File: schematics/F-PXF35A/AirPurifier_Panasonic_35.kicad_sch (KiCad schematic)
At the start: 63 parts, among them Q1 N6, Q2 N6, Q3 N6, Q4 N6, Q5 N6, Q7 N6, SW1 ON/OFF, SW2 AirVolume, SW3 Turbo, SW4 Sleep, U1 WEMOS_D1_mini, U2 PCF8575DBR, U3 PC847

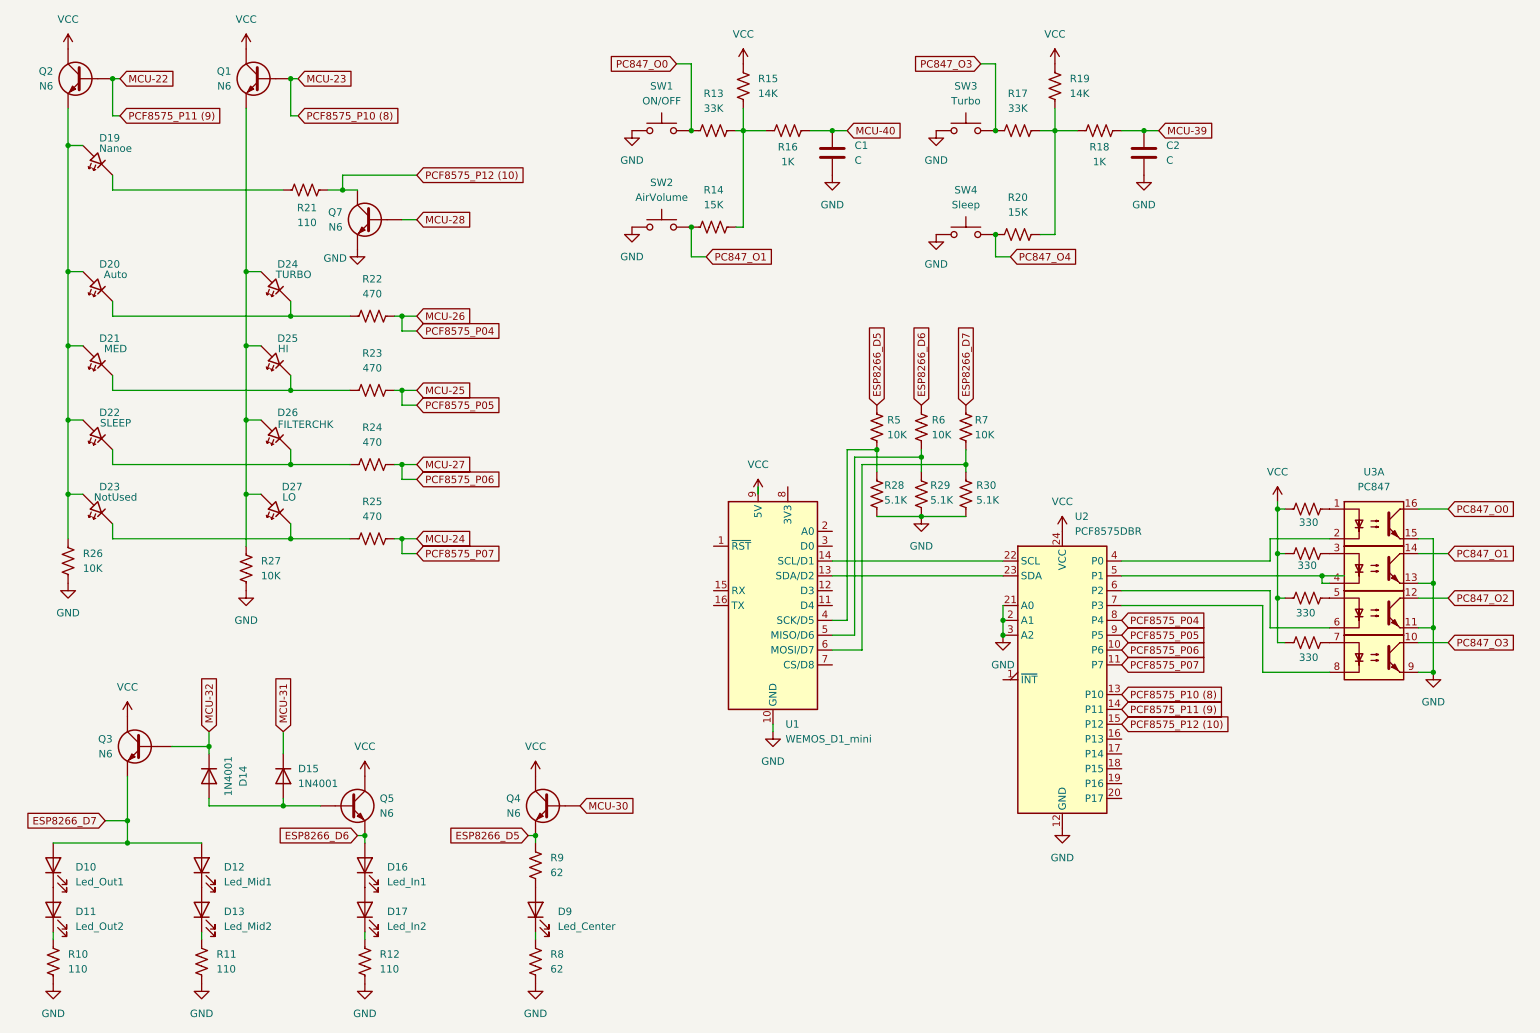
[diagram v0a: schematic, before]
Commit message: correct sch
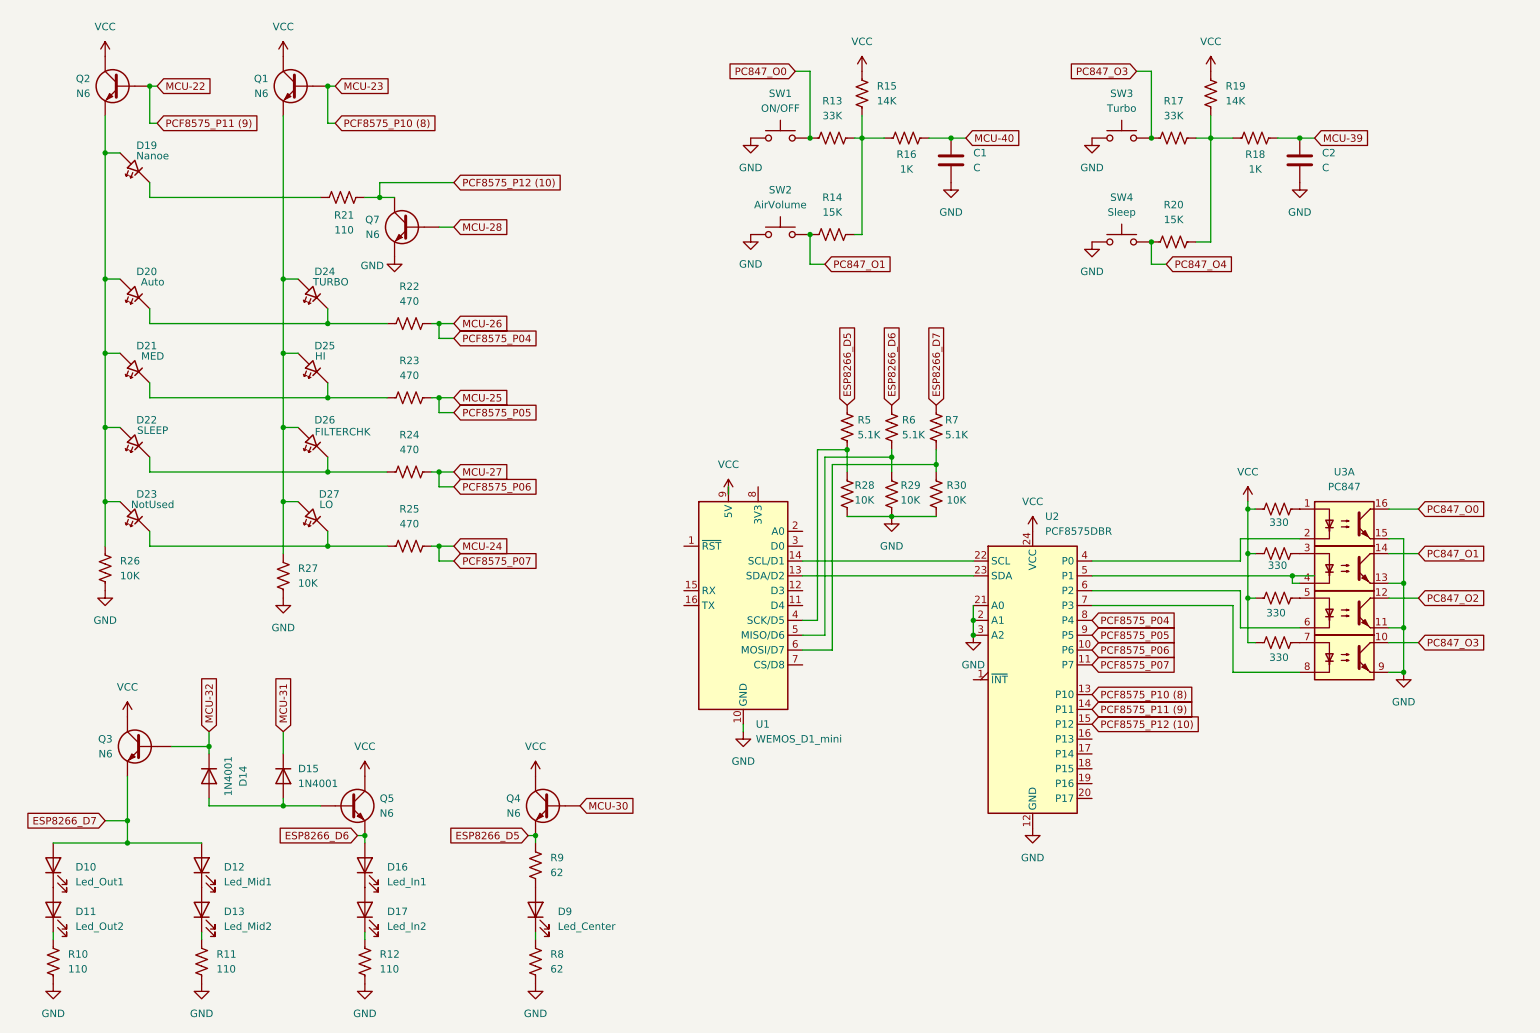
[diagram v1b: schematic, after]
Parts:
- R28, R29, R30: value 5.1K -> 10K
- R5, R6, R7: value 10K -> 5.1K
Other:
- moved on the sheet: C1, C2, D19, D20, D21, D22, D23, D24, D25, D26, D27, Q1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
